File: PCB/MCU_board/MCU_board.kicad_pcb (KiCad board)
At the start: 2 copper layers, 70 x 70 mm, 49 parts, among them IC1 NEO-F10N-00B, IC2 TXB0104PWR, IC3 ESP32-S3-WROOM-1-N4R8, IC6 4259-63, IC8 MAX98357AETE+T, J1 DS1013-40SSIB1-B-0, J4 FXP612 (u.FL) 2, J5 FXP612 (u.FL) 1, J6 SIM8055-6-1-14-00-A, J7 FXP612 (u.FL) 1, Q3 Si2323DDS-T1-GE3, Q4 BSS138, Q5 BSS138, U2 SIM7000G

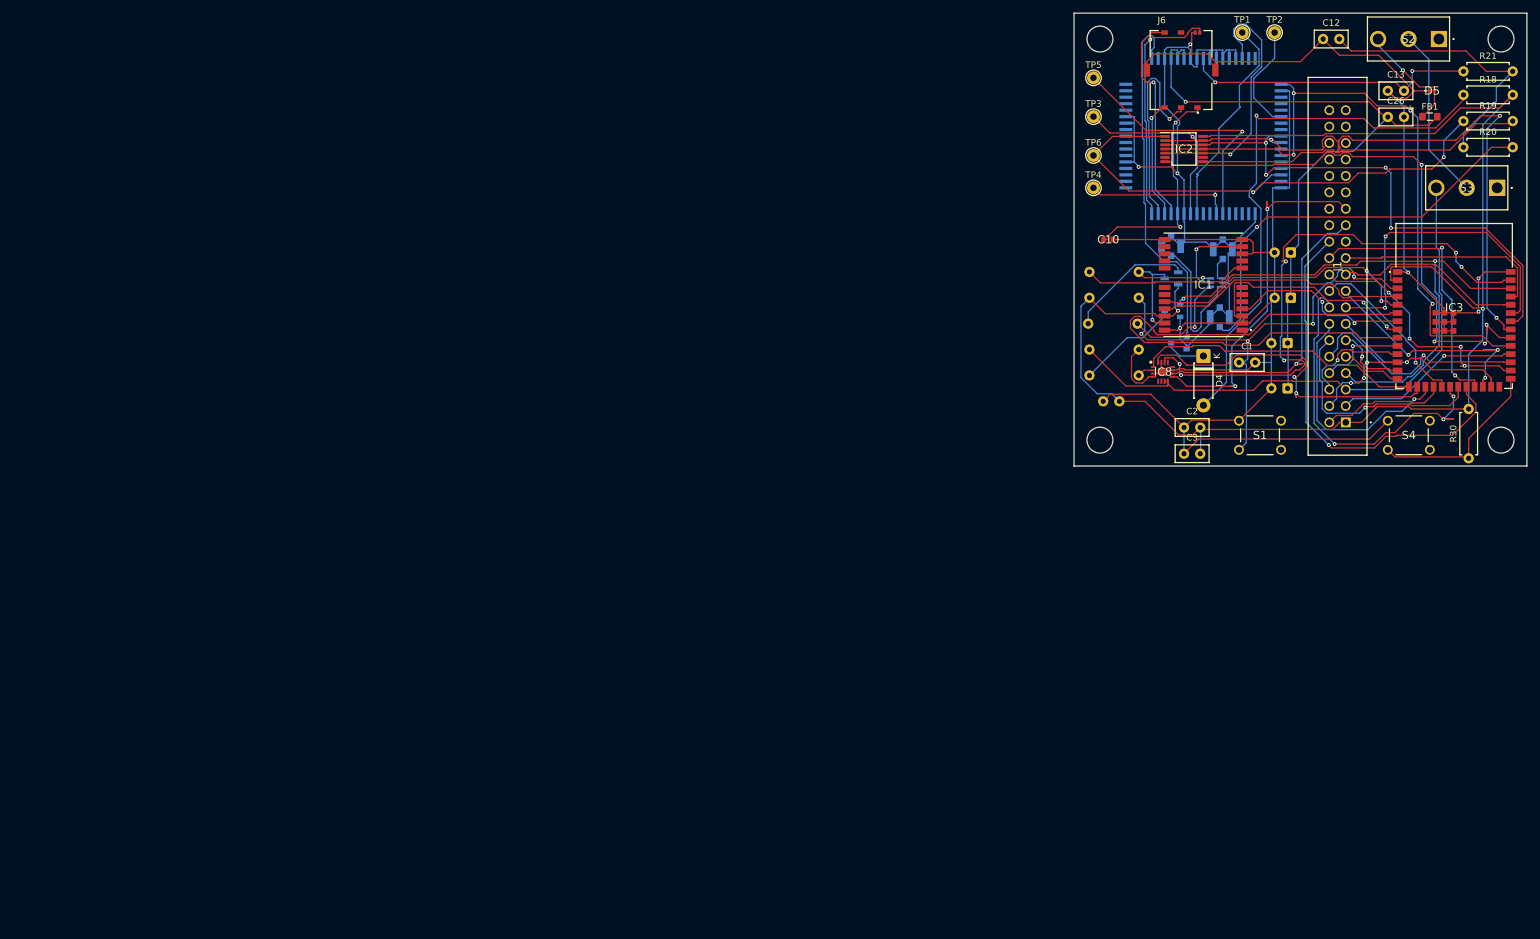
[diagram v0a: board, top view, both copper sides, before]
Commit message: routing on your own
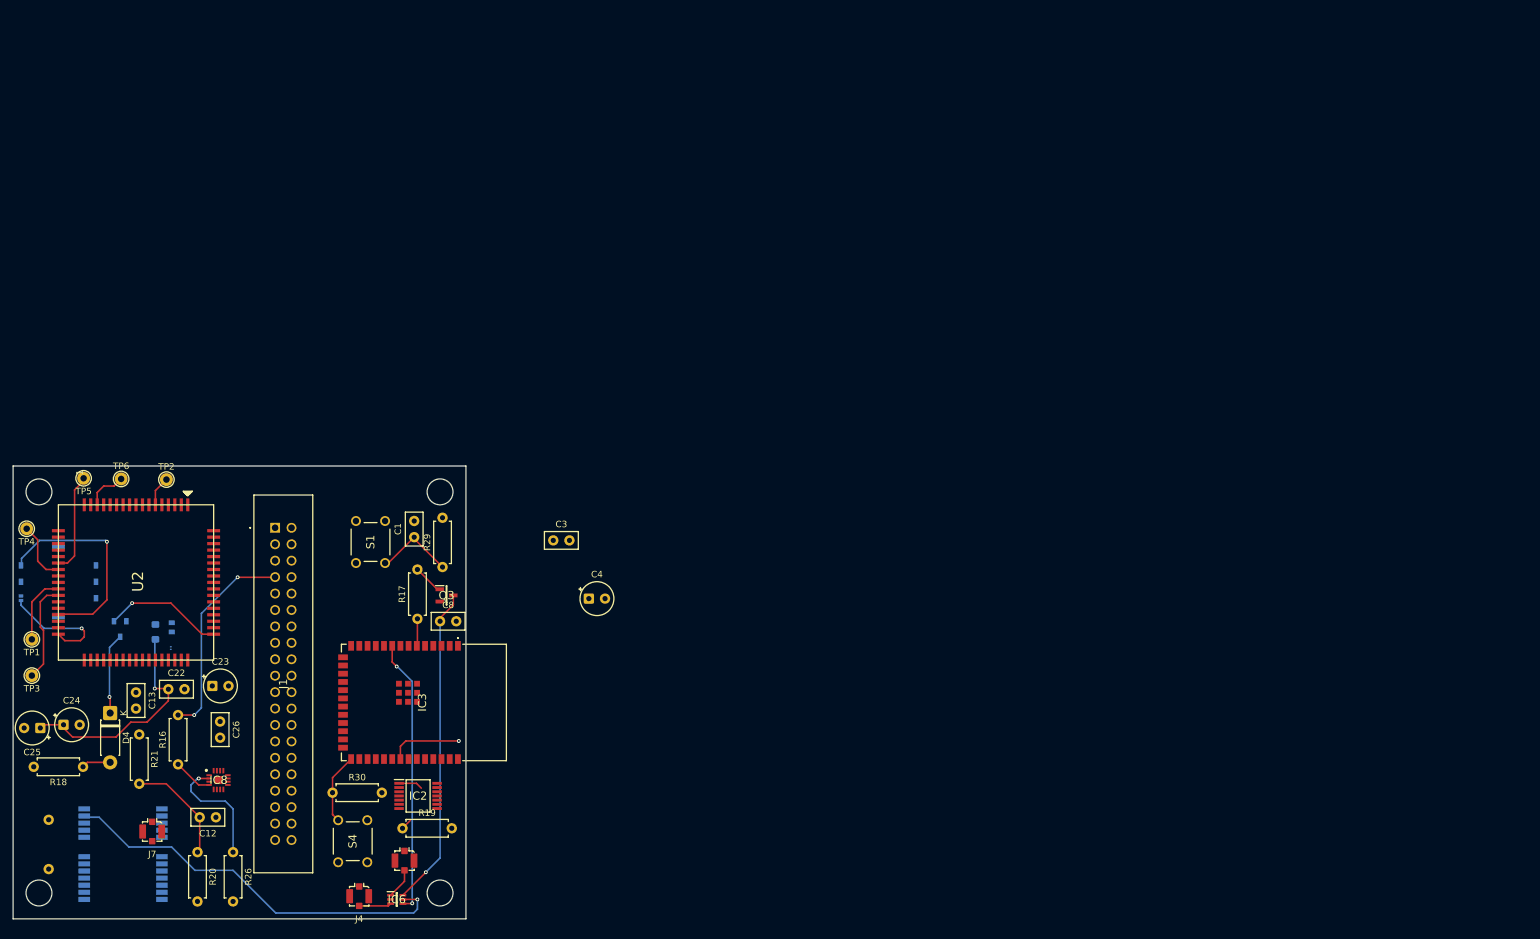
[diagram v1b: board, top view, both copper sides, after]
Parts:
- removed C2: 1μF, Capacitor_THT:C_Disc_D5.0mm_W2.5mm_P2.50mm
- removed D5: PESD3V3L1BSLZ, PESD3V3L1BSLZ:PESD3V3L1BSLZ
- removed Q4: BSS138, BSS138:SOT95P240X120-3N
- removed S2, S3: SLW-1276864-4A-D, SLW-1276864-4A-D:SLW12768644AD
- added C4: 1μF, Capacitor_THT:CP_Radial_Tantal_D5.0mm_P2.50mm, F.Cu at (119.0, 120.5)
- added D1: PESD5V0C1BSFYL, PESD5V0C1BSFYL:PMEG3005AESFYL, B.Cu at (54.4, 128.0)
- C1: value 100nF -> 1μF
- C10, FB1, IC1, J6: moved to B.Cu
- C22: footprint Capacitor_THT:CP_Radial_Tantal_D5.0mm_P2.50mm -> Capacitor_THT:C_Disc_D5.0mm_W2.5mm_P2.50mm; moved to F.Cu
- C23: value 100µF -> 1000µF; moved to F.Cu
- C24, C25, C8, IC6, J4, J5, J7, Q3, R17, R26, R29, U2: moved to F.Cu
- R16: value 680kΩ -> 100kΩ; moved to F.Cu
- moved R18 237.3 mm to (40.8, 146.5), turned to 180 degrees
- moved R21 228.9 mm to (49.5, 141.5), turned to -90 degrees
- moved R20 224.0 mm to (58.5, 159.7), turned to -90 degrees
- moved C13 214.7 mm to (49.0, 135.0), turned to -90 degrees
- moved FB1 212.5 mm to (52.0, 125.7), turned to -90 degrees
- moved TP1 209.3 mm to (32.9, 126.8), turned to 180 degrees
- moved C12 209.2 mm to (61.4, 154.3), turned to 180 degrees
- moved C26 203.3 mm to (62.0, 139.5), turned to -90 degrees
- moved C25 199.8 mm to (34.2, 140.5)
- moved C24 198.2 mm to (37.8, 140.0), turned to 0 degrees
- moved R19 197.1 mm to (90.2, 156.0)
- moved R28 192.1 mm to (35.5, 162.3), turned to 90 degrees
- moved J6 190.7 mm to (37.0, 117.9), turned to -90 degrees
- moved IC1 188.8 mm to (47.0, 160.0), turned to 180 degrees
- moved C22 186.2 mm to (54.0, 134.5), turned to 0 degrees
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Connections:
- C8 pad 1: /+3V3 -> Net-(IC1-VCC)
- FB1 pad 1: Net-(D5-K2) -> /3V8
- IC1 pad 22: /+3V3 -> Net-(IC1-VCC)
- J1 pad 26: unconnected-(J1-Pad26) -> /3V8
- R16 pad 2: /OUT+5V -> /LOUDNESS
- R26 pad 2: Net-(Q4-D) -> GND
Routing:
- net GND: track 437.6 -> 0.00 mm, vias 7 -> 0
- net /+3V3: track 224.6 -> 0.00 mm, vias 2 -> 0
- net /STATUS: track 130.3 -> 0.00 mm, vias 5 -> 0
- net /PWRKEY: track 104.2 -> 0.00 mm, vias 4 -> 0
- net /G_LRCLK: track 90.5 -> 0.00 mm, vias 6 -> 0
- net /OUT+5V: track 87.5 -> 0.00 mm
- net /GSM_RXT: track 98.1 -> 11.6 mm, vias 3 -> 1
- net /GSM_TXD: track 85.2 -> 0.00 mm, vias 4 -> 0
- net Net-(D4-A): track 85.1 -> 4.48 mm, vias 1 -> 0
- net /Stationary/GSM_sheet/OUT1.8V: track 83.3 -> 11.9 mm, vias 2 -> 0
- net Net-(U2-VBAT@1): track 105.8 -> 35.0 mm
- net /ACCEL_CS: track 64.7 -> 0.00 mm, vias 1 -> 0
- net Net-(IC3-EN): track 77.1 -> 12.6 mm, vias 4 -> 0
- net Net-(J7-In): track 64.1 -> 0.00 mm, vias 1 -> 0
- net /OUT_P: track 59.5 -> 0.00 mm, vias 2 -> 0
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- added copper zone on In1.Cu, net /+3V3
- added copper zone on In2.Cu, net GND
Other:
- copper layers 2 -> 4
